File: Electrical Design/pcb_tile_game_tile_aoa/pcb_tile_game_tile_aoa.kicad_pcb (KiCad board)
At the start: 2 copper layers, 69.3 x 60 mm, 40 parts, among them J1 Conn_01x05_Pin, J2 Conn_01x05_Socket, J3 Conn_01x05_Pin, J4 Conn_01x05_Socket, J5 Conn_01x05_Pin, J6 Conn_01x05_Socket, U2 ATtiny3217-M

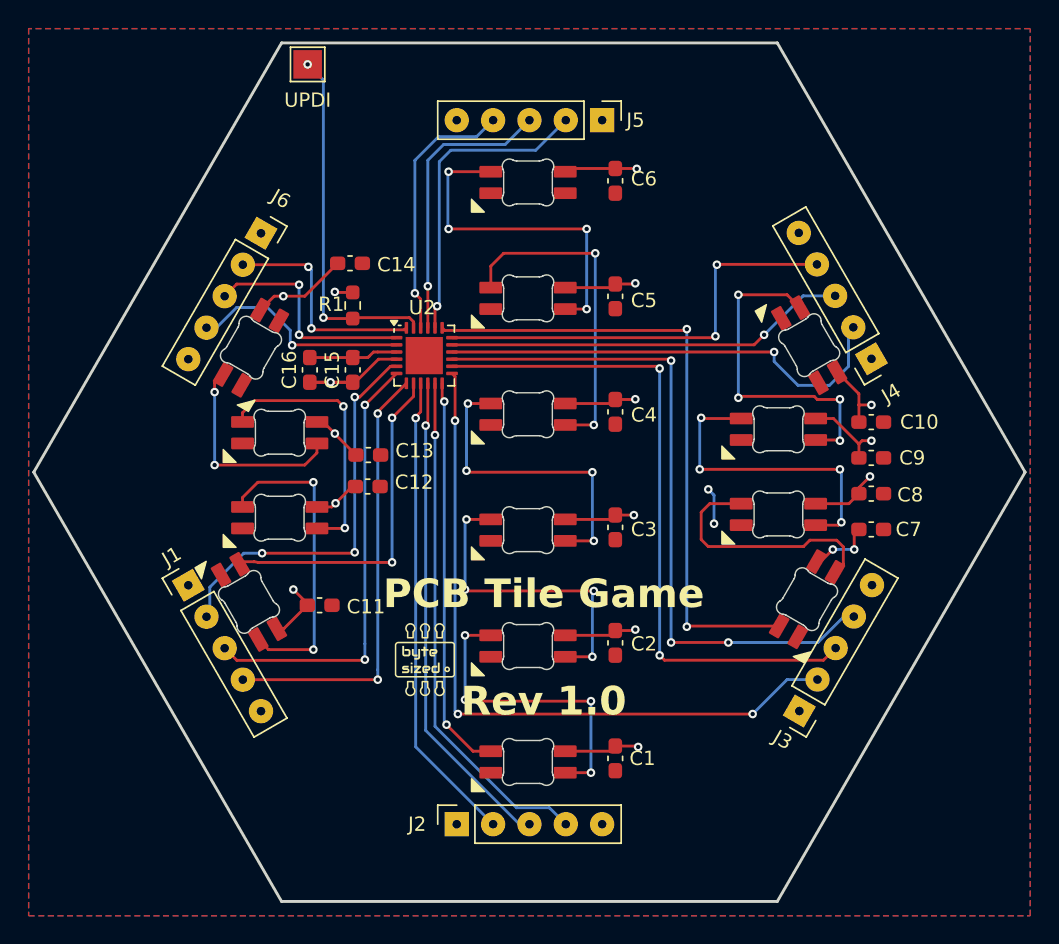
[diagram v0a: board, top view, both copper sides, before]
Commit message: created gerbers
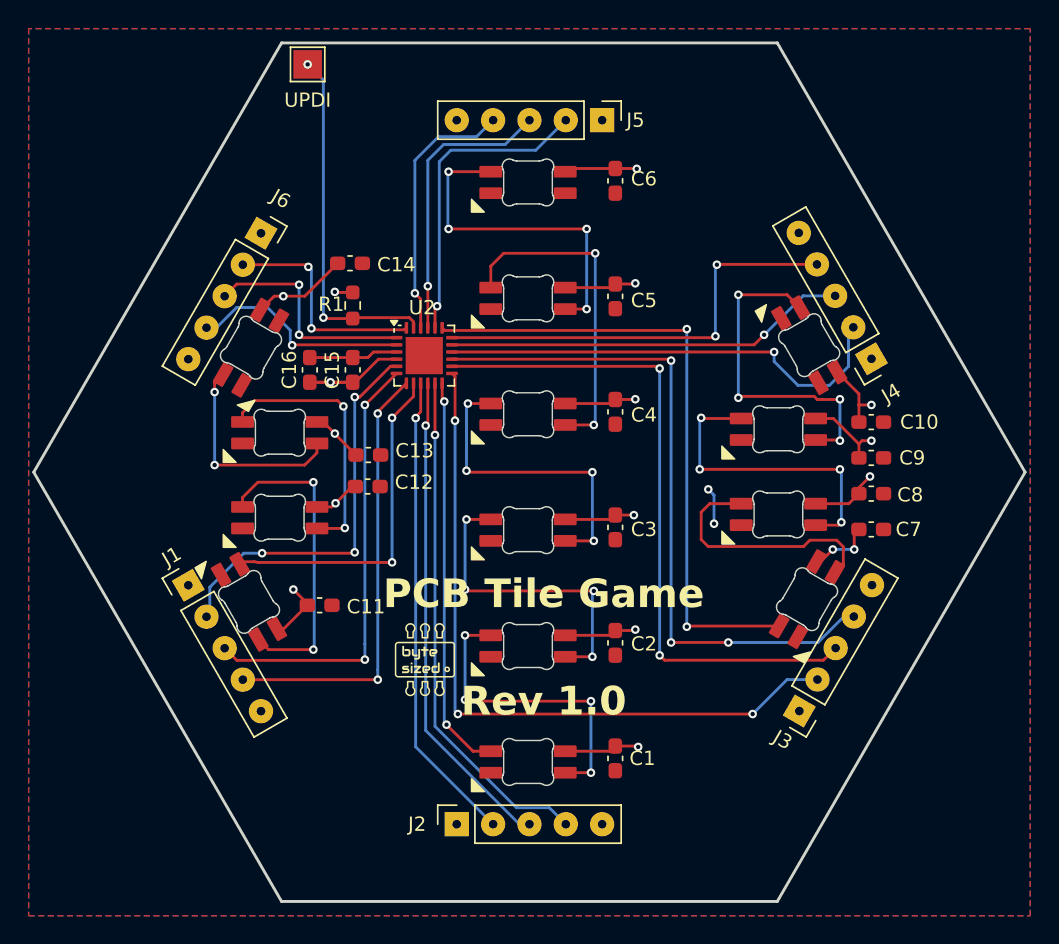
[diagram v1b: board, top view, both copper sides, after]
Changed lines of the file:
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@@
 			(drillshape 0)
 			(scaleselection 1)
-			(outputdirectory "")
+			(outputdirectory "aoa.gerbers/")
 		)
 	)
@@
 		(fp_arc
 			(start 1.699999 -0.990938)
-			(mid 1.712519 -1.102166)
+			(mid 1.712521 -1.102165)
 			(end 1.749484 -1.207816)
 			(stroke
@@
 		(fp_arc
 			(start 1.046711 -1.856395)
-			(mid 1.638074 -1.79213)
+			(mid 1.63807 -1.792132)
 			(end 1.749484 -1.207815)
 			(stroke
@@
 		(fp_arc
 			(start 1.046711 -1.856395)
-			(mid 0.925123 -1.805473)
+			(mid 0.925123 -1.805472)
 			(end 0.794452 -1.788096)
 			(stroke
@@
 		(fp_arc
 			(start 1.699999 -0.990938)
-			(mid 1.712519 -1.102166)
+			(mid 1.712521 -1.102165)
 			(end 1.749484 -1.207816)
 			(stroke
@@
 		(fp_arc
 			(start 1.046711 -1.856395)
-			(mid 1.638074 -1.79213)
+			(mid 1.63807 -1.792132)
 			(end 1.749484 -1.207815)
 			(stroke
@@
 		(fp_arc
 			(start 1.046711 -1.856395)
-			(mid 0.925123 -1.805473)
+			(mid 0.925123 -1.805472)
 			(end 0.794452 -1.788096)
 			(stroke
@@
 		(fp_arc
 			(start 1.04671 -1.856396)
-			(mid 0.925122 -1.805472)
+			(mid 0.925123 -1.805473)
 			(end 0.794452 -1.788094)
 			(stroke
@@
 		(fp_arc
 			(start 1.04671 -1.856396)
-			(mid 1.638075 -1.792131)
+			(mid 1.63807 -1.792133)
 			(end 1.749484 -1.207815)
 			(stroke
@@
 		(fp_arc
 			(start 0.794452 1.211902)
-			(mid 0.925124 1.229278)
+			(mid 0.925124 1.229279)
 			(end 1.046712 1.280204)
 			(stroke
@@
 		(fp_arc
 			(start 1.699999 -0.990938)
-			(mid 1.712519 -1.102166)
+			(mid 1.712521 -1.102165)
 			(end 1.749484 -1.207816)
 			(stroke
@@
 		(fp_arc
 			(start 1.046711 -1.856395)
-			(mid 1.638074 -1.79213)
+			(mid 1.63807 -1.792132)
 			(end 1.749484 -1.207815)
 			(stroke
@@
 		(fp_arc
 			(start 1.046711 -1.856395)
-			(mid 0.925123 -1.805473)
+			(mid 0.925123 -1.805472)
 			(end 0.794452 -1.788096)
 			(stroke
@@
 		(fp_arc
 			(start 1.699999 -0.990938)
-			(mid 1.712519 -1.102166)
+			(mid 1.712521 -1.102165)
 			(end 1.749484 -1.207816)
 			(stroke
@@
 		(fp_arc
 			(start 1.046711 -1.856395)
-			(mid 1.638074 -1.79213)
+			(mid 1.63807 -1.792132)
 			(end 1.749484 -1.207815)
 			(stroke
@@
 		(fp_arc
 			(start 1.046711 -1.856395)
-			(mid 0.925123 -1.805473)
+			(mid 0.925123 -1.805472)
 			(end 0.794452 -1.788096)
 			(stroke
@@
 		(fp_arc
 			(start 1.699999 -0.990938)
-			(mid 1.712519 -1.102166)
+			(mid 1.712521 -1.102165)
 			(end 1.749484 -1.207816)
 			(stroke
@@
 		(fp_arc
 			(start 1.046711 -1.856395)
-			(mid 1.638074 -1.79213)
+			(mid 1.63807 -1.792132)
 			(end 1.749484 -1.207815)
 			(stroke
@@
 		(fp_arc
 			(start 1.046711 -1.856395)
-			(mid 0.925123 -1.805473)
+			(mid 0.925123 -1.805472)
 			(end 0.794452 -1.788096)
 			(stroke
@@
 		(fp_arc
 			(start 0.794452 1.211902)
-			(mid 0.925123 1.22928)
+			(mid 0.925123 1.229281)
 			(end 1.046712 1.280202)
 			(stroke
@@
 		(fp_arc
 			(start 1.749483 0.631624)
-			(mid 1.712547 0.525969)
+			(mid 1.712554 0.525967)
 			(end 1.7 0.414748)
 			(stroke
@@
 		(fp_arc
 			(start -1.046712 1.280204)
-			(mid -1.638069 1.215936)
+			(mid -1.638069 1.215935)
 			(end -1.749484 0.631623)
 			(stroke
@@
 		(fp_arc
 			(start -1.749485 -1.207816)
-			(mid -1.712524 -1.102165)
+			(mid -1.712523 -1.102165)
 			(end -1.699999 -0.990938)
 			(stroke
@@
 		(fp_arc
 			(start 1.699999 -0.990938)
-			(mid 1.712519 -1.102166)
+			(mid 1.712521 -1.102165)
 			(end 1.749484 -1.207816)
 			(stroke
@@
 		(fp_arc
 			(start 1.046711 -1.856395)
-			(mid 1.638074 -1.79213)
+			(mid 1.63807 -1.792132)
 			(end 1.749484 -1.207815)
 			(stroke
@@
 		(fp_arc
 			(start 1.046711 -1.856395)
-			(mid 0.925123 -1.805473)
+			(mid 0.925123 -1.805472)
 			(end 0.794452 -1.788096)
 			(stroke
@@
 		(fp_arc
 			(start 1.046711 -1.856395)
-			(mid 0.925123 -1.805471)
+			(mid 0.925124 -1.805471)
 			(end 0.794452 -1.788097)
 			(stroke
@@
 		(fp_arc
 			(start 1.046711 -1.856395)
-			(mid 1.638074 -1.79213)
+			(mid 1.63807 -1.792132)
 			(end 1.749484 -1.207815)
 			(stroke
@@
 		(fp_arc
 			(start 1.699999 -0.990938)
-			(mid 1.712519 -1.102166)
+			(mid 1.712521 -1.102165)
 			(end 1.749484 -1.207816)
 			(stroke
@@
 		(fp_arc
 			(start 1.046711 -1.856395)
-			(mid 1.638074 -1.79213)
+			(mid 1.63807 -1.792132)
 			(end 1.749484 -1.207815)
 			(stroke
@@
 		(fp_arc
 			(start 1.046711 -1.856395)
-			(mid 0.925123 -1.805473)
+			(mid 0.925123 -1.805472)
 			(end 0.794452 -1.788096)
 			(stroke
@@
 		(fp_arc
 			(start 1.699999 -0.990938)
-			(mid 1.712519 -1.102166)
+			(mid 1.712521 -1.102165)
 			(end 1.749484 -1.207816)
 			(stroke
@@
 		(fp_arc
 			(start 1.046711 -1.856395)
-			(mid 1.638074 -1.79213)
+			(mid 1.63807 -1.792132)
 			(end 1.749484 -1.207815)
 			(stroke
@@
 		(fp_arc
 			(start 1.046711 -1.856395)
-			(mid 0.925123 -1.805473)
+			(mid 0.925123 -1.805472)
 			(end 0.794452 -1.788096)
 			(stroke
@@
 		(fp_arc
 			(start 1.699999 -0.990938)
-			(mid 1.712519 -1.102166)
+			(mid 1.712521 -1.102165)
 			(end 1.749484 -1.207816)
 			(stroke
@@
 		(fp_arc
 			(start 1.046711 -1.856395)
-			(mid 1.638074 -1.79213)
+			(mid 1.63807 -1.792132)
 			(end 1.749484 -1.207815)
 			(stroke
@@
 		(fp_arc
 			(start 1.046711 -1.856395)
-			(mid 0.925123 -1.805473)
+			(mid 0.925123 -1.805472)
 			(end 0.794452 -1.788096)
 			(stroke
@@
 		(fp_arc
 			(start 1.699999 -0.990938)
-			(mid 1.712519 -1.102166)
+			(mid 1.712521 -1.102165)
 			(end 1.749484 -1.207816)
 			(stroke
@@
 		(fp_arc
 			(start 1.046711 -1.856395)
-			(mid 1.638074 -1.79213)
+			(mid 1.63807 -1.792132)
 			(end 1.749484 -1.207815)
 			(stroke
@@
 		(fp_arc
 			(start 1.046711 -1.856395)
-			(mid 0.925123 -1.805473)
+			(mid 0.925123 -1.805472)
 			(end 0.794452 -1.788096)
 			(stroke
